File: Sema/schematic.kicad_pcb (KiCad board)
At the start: 2 copper layers, 98.8 x 91 mm, 80 parts, among them J1 Conn_01x05_Male, J10 Conn_01x05_Male, J11 Conn_01x05_Male, J12 Conn_01x05_Male, J3 Conn_01x03_Male, J4 Conn_01x05_Male, J5 Conn_01x03_Male, J7 Conn_01x05_Male, J8 Conn_01x05_Male, J9 Conn_01x05_Male, U1 LM317AT/NOPB, U10 74LVT573MTC, U11 74LVT573MTC, U12 74LVT573MTC, U13 74LVT573MTC, U14 ULN2003AIDR, U15 ULN2003AIDR, U16 ULN2003AIDR, U17 ULN2003AIDR, U2 LM317AT/NOPB, U3 PIC24FJ64GA702-I/SO, U4 ABLS-8.000MHZ-B2-T, U5 FT232RL, U6 CD74HC4514M96, U7 PTMUX1308QDYYRQ1, U8 74LVT573MTC, U9 74LVT573MTC

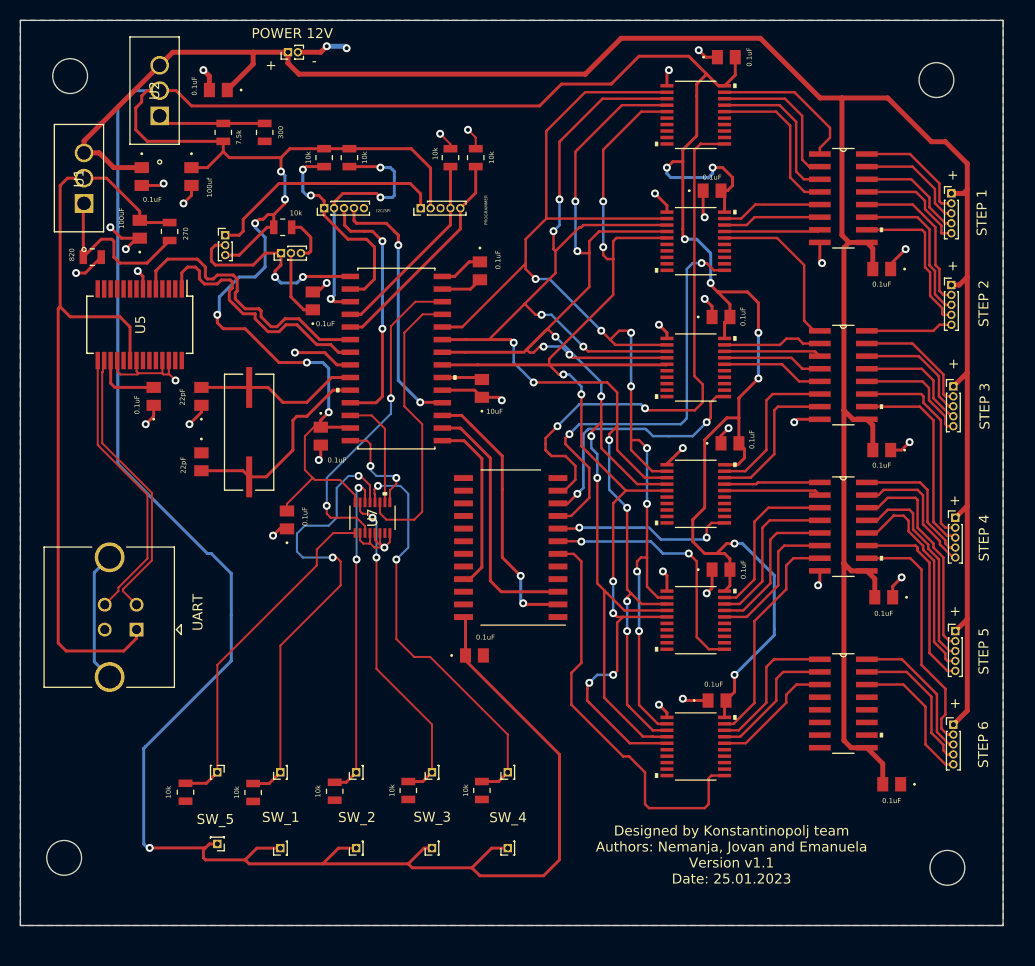
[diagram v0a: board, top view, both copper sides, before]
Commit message: Izmjene na layout-u
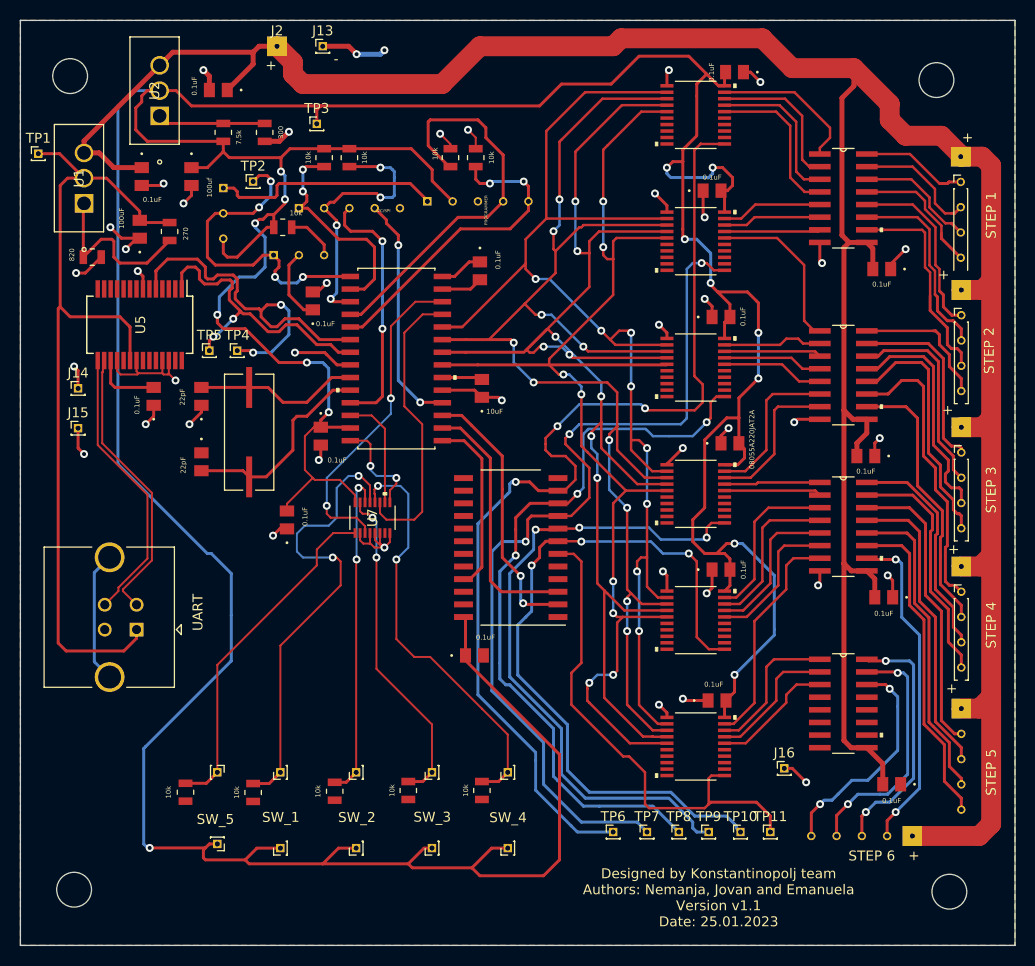
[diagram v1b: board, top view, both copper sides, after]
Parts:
- removed POWER 12V: Conn_01x02_Male, Connector_PinHeader_1.00mm:PinHeader_1x02_P1.00mm_Vertical
- added J13: Conn_01x01_Male, Connector_PinHeader_1.00mm:PinHeader_1x01_P1.00mm_Vertical, F.Cu at (78.6, 39.6)
- added J14: Conn_01x01_Male, Connector_PinHeader_1.00mm:PinHeader_1x01_P1.00mm_Vertical, F.Cu at (54.0, 74.0)
- added J15: Conn_01x01_Male, Connector_PinHeader_1.00mm:PinHeader_1x01_P1.00mm_Vertical, F.Cu at (54.0, 78.0)
- added J16: Conn_01x01_Male, Connector_PinHeader_1.00mm:PinHeader_1x01_P1.00mm_Vertical, F.Cu at (125.0, 112.2)
- added J2: Conn_01x01_Male, Connector_PinHeader_1.00mm:PinHeader_1x01_P1.00mm_Vertical, F.Cu at (74.0, 39.6)
- added TP1: TestPoint, Connector_PinHeader_1.00mm:PinHeader_1x01_P1.00mm_Vertical, F.Cu at (50.0, 50.4)
- added TP10: TestPoint, Connector_PinHeader_1.00mm:PinHeader_1x01_P1.00mm_Vertical, F.Cu at (120.6, 118.6)
- added TP11: TestPoint, Connector_PinHeader_1.00mm:PinHeader_1x01_P1.00mm_Vertical, F.Cu at (123.6, 118.6)
- added TP2: TestPoint, Connector_PinHeader_1.00mm:PinHeader_1x01_P1.00mm_Vertical, F.Cu at (71.6, 53.2)
- added TP3: TestPoint, Connector_PinHeader_1.00mm:PinHeader_1x01_P1.00mm_Vertical, F.Cu at (78.0, 47.4)
- added TP4: TestPoint, Connector_PinHeader_1.00mm:PinHeader_1x01_P1.00mm_Vertical, F.Cu at (70.0, 70.2)
- added TP5: TestPoint, Connector_PinHeader_1.00mm:PinHeader_1x01_P1.00mm_Vertical, F.Cu at (67.2, 70.2)
- added TP6: TestPoint, Connector_PinHeader_1.00mm:PinHeader_1x01_P1.00mm_Vertical, F.Cu at (107.8, 118.6)
- added TP7: TestPoint, Connector_PinHeader_1.00mm:PinHeader_1x01_P1.00mm_Vertical, F.Cu at (111.2, 118.6)
- added TP8: TestPoint, Connector_PinHeader_1.00mm:PinHeader_1x01_P1.00mm_Vertical, F.Cu at (114.4, 118.6)
- added TP9: TestPoint, Connector_PinHeader_1.00mm:PinHeader_1x01_P1.00mm_Vertical, F.Cu at (117.4, 118.6)
- 0.1uF1: value 0.1uF -> 08055A220JAT2A
- moved J11 13.0 mm to (135.3, 119.0), turned to -90 degrees
- moved J10 11.6 mm to (142.8, 110.0)
- moved J12 7.47 mm to (142.8, 94.4)
- moved J9 6.69 mm to (142.8, 80.4)
- moved H4 3.35 mm to (53.6, 124.4)
- moved J4 3.29 mm to (91.7, 55.2)
- moved J8 3.20 mm to (142.8, 66.6)
- moved H3 2.41 mm to (141.6, 124.6)
- moved J3 2.21 mm to (68.6, 56.4)
- moved J5 1.81 mm to (76.2, 60.6)
- moved C14 1.71 mm to (120.0, 42.2), turned to 180 degrees
- moved C20 1.71 mm to (133.2, 80.8)
- moved J7 1.49 mm to (142.7, 53.2)
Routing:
- net E1: track 55.3 -> 104.6 mm, vias 2 -> 3
- net E3: track 25.9 -> 74.8 mm, vias 2 -> 3
- net E4: track 18.6 -> 66.2 mm, vias 2 -> 3
- net E5: track 25.7 -> 73.3 mm, vias 2 -> 3
- net E2: track 43.3 -> 90.5 mm, vias 2 -> 3
- net 12V: track 267.7 -> 299.1 mm
- net PGD: track 19.7 -> 39.9 mm
- net B3: track 11.7 -> 24.7 mm
- net B5: track 19.6 -> 32.5 mm
- net GND: track 109.5 -> 121.5 mm, vias 38 -> 42
- net Net-(J3-Pad2): track 21.2 -> 33.0 mm, vias 2 -> 4
- net tx: track 28.6 -> 40.3 mm, vias 0 -> 2
- net PI3: track 11.7 -> 23.2 mm
- net Y6: track 14.5 -> 25.1 mm, vias 0 -> 2
- net PI6: track 14.6 -> 25.0 mm, vias 0 -> 2
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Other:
- board size 98.8 x 91 mm -> 100 x 93 mm
